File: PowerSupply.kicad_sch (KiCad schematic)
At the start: 17 parts, among them U3 nPM1100-CAXX, U6 TPS62173DSG, U9 TPS22917DBV

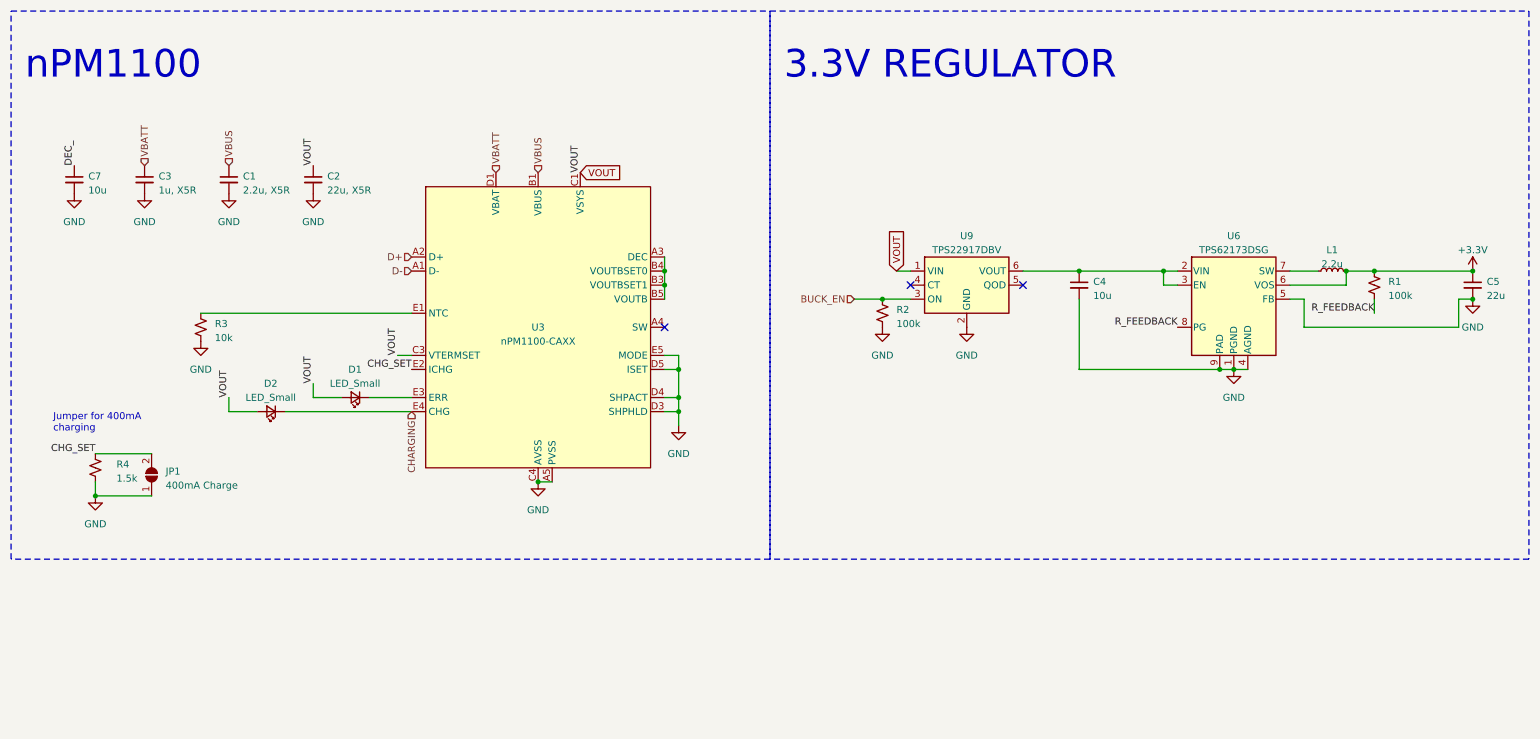
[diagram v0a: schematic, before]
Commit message: Schematic complete.
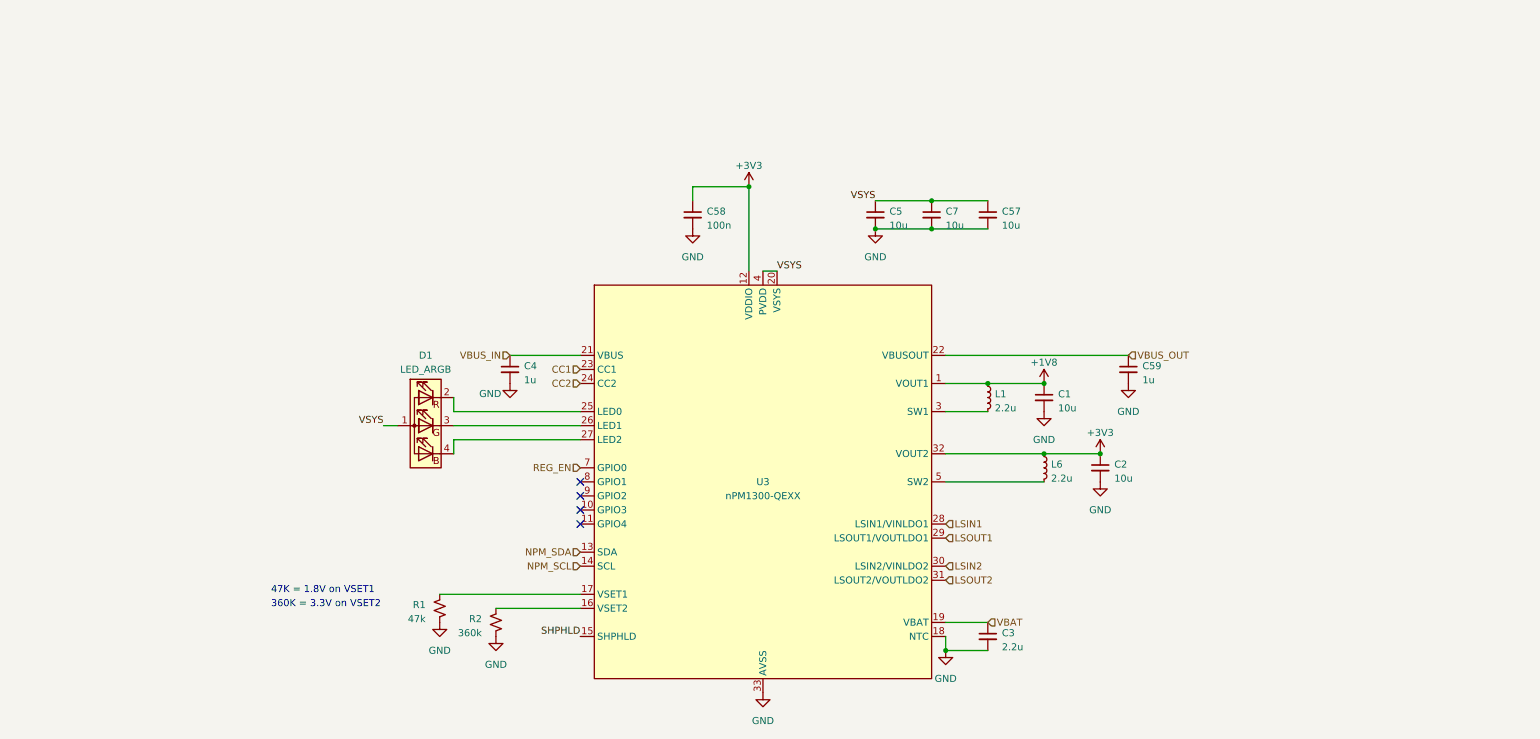
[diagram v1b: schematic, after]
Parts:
- removed D1, D2: LED_Small, symbol Device:LED_Small
- removed JP1: 400mA Charge, Jumper:SolderJumper-2_P1.3mm_Open_RoundedPad1.0x1.5mm, symbol Jumper:SolderJumper_2_Open
- removed R3: 10k, symbol Device:R_Small_US
- removed R4: 1.5k, symbol Device:R_Small_US
- removed U3: nPM1100-CAXX, nordic-lib-kicad-npm:BGA-25_5x5_2.075x2.075mm, symbol nordic-lib-kicad-npm:nPM1100-CAXX
- removed U6: TPS62173DSG, Package_SON:WSON-8-1EP_2x2mm_P0.5mm_EP0.9x1.6mm_ThermalVias, symbol Regulator_Switching:TPS62173DSG
- removed U9: TPS22917DBV, Package_TO_SOT_SMD:SOT-23-6, symbol Power_Management:TPS22917DBV
- added C57: 10u, Capacitor_SMD:C_0402_1005Metric, symbol Device:C_Small
- added C58: 100n, Capacitor_SMD:C_0402_1005Metric, symbol Device:C_Small
- added C59: 1u, Capacitor_SMD:C_0402_1005Metric, symbol Device:C_Small
- added D1: LED_ARGB, LED_SMD:LED_SK6812_EC15_1.5x1.5mm, symbol Device:LED_ARGB
- added L6: 2.2u, Inductor_SMD:L_0805_2012Metric, symbol Device:L_Small
- added U3: nPM1300-QEXX, Package_DFN_QFN:QFN-32-1EP_5x5mm_P0.5mm_EP3.6x3.6mm_ThermalVias, symbol nordic-lib-kicad-npm:nPM1300-QEXX
- C1: value 2.2u, X5R -> 10u; footprint (none) -> Capacitor_SMD:C_0402_1005Metric
- C2: value 22u, X5R -> 10u; footprint (none) -> Capacitor_SMD:C_0402_1005Metric
- C3: value 1u, X5R -> 2.2u; footprint (none) -> Capacitor_SMD:C_0402_1005Metric
- C4: value 10u -> 1u; footprint (none) -> Capacitor_SMD:C_0402_1005Metric
- C5: value 22u -> 10u; footprint (none) -> Capacitor_SMD:C_0402_1005Metric
- C7: footprint (none) -> Capacitor_SMD:C_0402_1005Metric
- L1: footprint (none) -> Inductor_SMD:L_0805_2012Metric
- R1: value 100k -> 47k; footprint (none) -> Resistor_SMD:R_0603_1608Metric
- R2: value 100k -> 360k; footprint (none) -> Resistor_SMD:R_0603_1608Metric
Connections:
- net R_FEEDBACK is gone; now on net GND: R1.2
- net VBUS is gone; now on net +1V8: C1.1
- net GND: now also C57.2, C58.2, C59.2, U3.18 (NTC), U3.2 (PVSS1), U3.33 (AVSS), U3.6 (PVSS2)
- net VBUS_IN: now reaches C4.1
- net VBUS_IN: now also U3.21 (VBUS)
- net +1V8: now reaches L1.1
- net +1V8: now also U3.1 (VOUT1)
- removed net +3.3V: C5.1, L1.2, R1.1
- net BUCK_EN: no longer names the net of R2.1
- net BUCK_EN: now also U3.16 (VSET2)
- net DEC_ renamed VSYS
- net VSYS: now also C5.1, C57.1, D1.1 (A), U3.20 (VSYS), U3.4 (PVDD)
- net VBATT renamed VBAT
- net VBAT: now also U3.19 (VBAT)
- net VOUT renamed +3V3
- net +3V3: now also C58.1, L6.1, U3.12 (VDDIO), U3.32 (VOUT2)
- new net: R1.1, U3.17 (VSET1)
- new net: D1.2 (RK), U3.25 (LED0)
- new net: D1.3 (GK), U3.26 (LED1)
- new net: D1.4 (BK), U3.27 (LED2)
- new net: L1.2, U3.3 (SW1)
- new net: L6.2, U3.5 (SW2)
- new net CC1: U3.23 (CC1)
- new net CC2: U3.24 (CC2)
- new net LSIN1: U3.28 (LSIN1/VINLDO1)
- new net LSIN2: U3.30 (LSIN2/VINLDO2)
- new net LSOUT1: U3.29 (LSOUT1/VOUTLDO1)
- new net LSOUT2: U3.31 (LSOUT2/VOUTLDO2)
- new net NPM_SCL: U3.14 (SCL)
- new net NPM_SDA: U3.13 (SDA)
- new net REG_EN: U3.7 (GPIO0)
- new net SHPHLD: U3.15 (SHPHLD)
- new net VBUS_OUT: C59.1, U3.22 (VBUSOUT)
- no-connect marks 3 -> 4
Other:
- note added: "360K = 3.3V on VSET2"
- note added: "47K = 1.8V on VSET1"
- note removed: "3.3V REGULATOR"
- note removed: "Jumper for 400mA charging"
- note removed: "nPM1100"
